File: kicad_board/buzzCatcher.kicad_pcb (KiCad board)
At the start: 2 copper layers, 63 x 100 mm, 31 parts, among them IC1 CD4043BE-NG, IC2 COM-16473, IC3 CD74HCT173E, IC4 CD4072BE, IC5 SN74LS04N, IC6 SN74LS21NE4, IC7 TS02-66-60-BK-100-SCR-D, J1 154-UL6661, J2 154-UL6661, J3 154-UL6661, J4 154-UL6661, J5 USB4130-GF-C, Q1 BS170

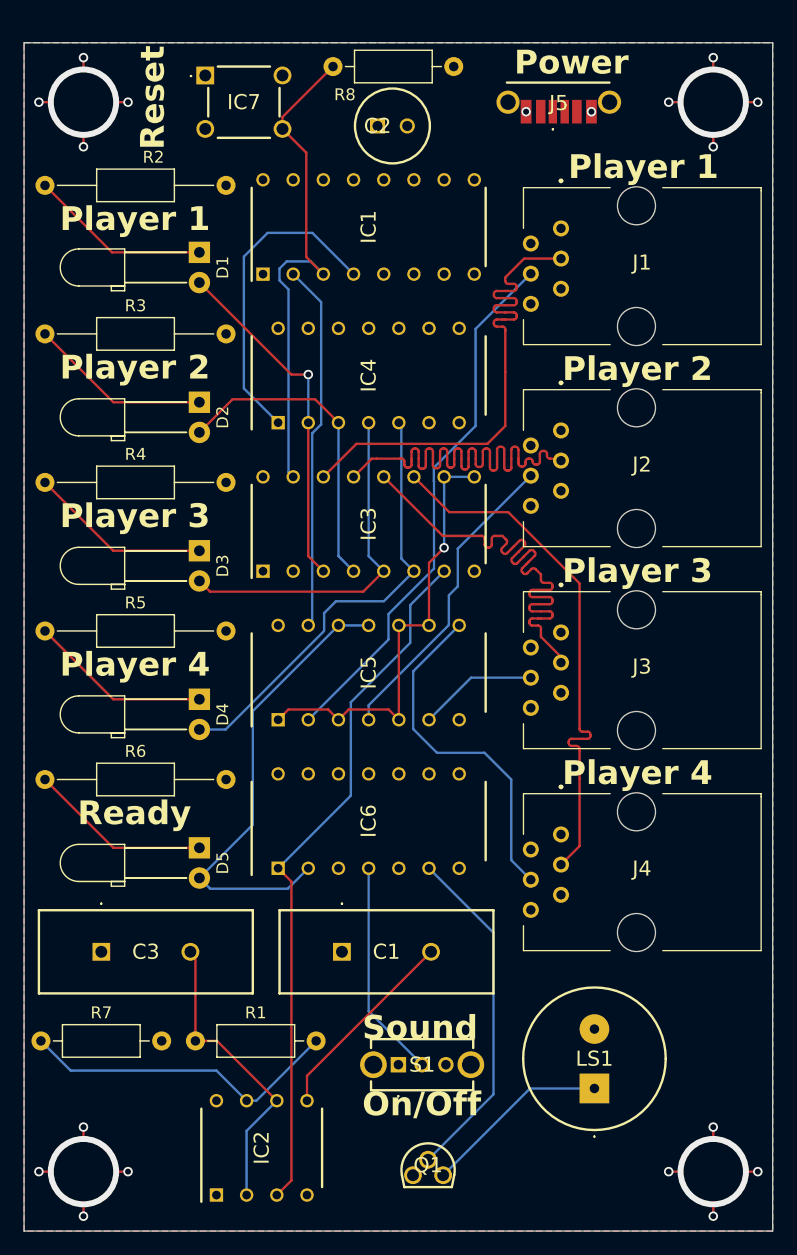
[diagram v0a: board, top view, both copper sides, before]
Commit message: Arduino version
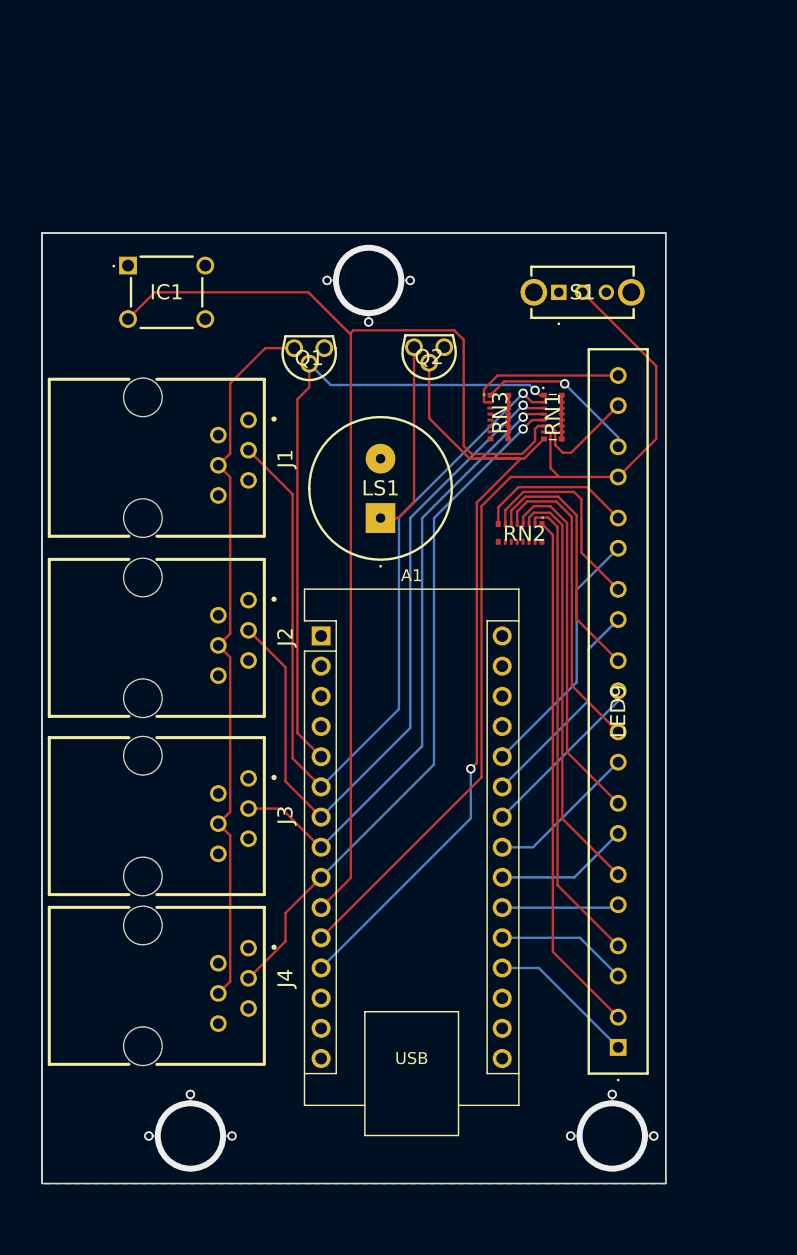
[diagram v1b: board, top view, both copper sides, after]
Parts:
- removed C1, C3: 3.3 nF, SamacSys_PCB_Library:ECWH16362RJV
- removed C2: 10 uF, SamacSys_PCB_Library:CAPPRD250W65D630H900
- removed D1, D2, D3, D4, D5: LED, LED_THT:LED_D3.0mm_Horizontal_O6.35mm_Z2.0mm
- removed IC2: COM-16473, SamacSys_PCB_Library:DIP794W53P254L959H508Q8N
- removed IC3: CD74HCT173E, SamacSys_PCB_Library:DIP794W53P254L1930H508Q16N
- removed IC4: CD4072BE, SamacSys_PCB_Library:DIP794W53P254L1930H508Q14N
- removed IC5: SN74LS04N, SamacSys_PCB_Library:DIP794W53P254L1930H508Q14N
- removed IC6: SN74LS21NE4, SamacSys_PCB_Library:DIP794W53P254L1930H508Q14N
- removed IC7: TS02-66-60-BK-100-SCR-D, SamacSys_PCB_Library:TS026660BK100SCRD
- removed J5: USB4130-GF-C, SamacSys_PCB_Library:USB4130GFC
- removed R1, R8: 110k, Resistor_THT:R_Axial_DIN0207_L6.3mm_D2.5mm_P10.16mm_Horizontal
- removed R2, R3, R4, R5, R6: 300, Resistor_THT:R_Axial_DIN0207_L6.3mm_D2.5mm_P15.24mm_Horizontal
- removed R7: 0, Resistor_THT:R_Axial_DIN0207_L6.3mm_D2.5mm_P10.16mm_Horizontal
- added A1: Arduino_Nano_v3.x, Module:Arduino_Nano, F.Cu at (75.0, 99.9)
- added LED9: SSA-LXH1025GD, SamacSys_PCB_Library:SSALXH1025GD, F.Cu at (100.0, 134.5)
- added Q2: BS170, SamacSys_PCB_Library:LM431ACZ, F.Cu at (85.4, 75.6)
- added RN1: EXB2HV103JV, SamacSys_PCB_Library:EXB2HV104JV, F.Cu at (94.5, 81.5)
- added RN2: EXB2HV121JV, SamacSys_PCB_Library:EXB2HV_1, F.Cu at (91.7, 91.3)
- added RN3: EXB2HV121JV, SamacSys_PCB_Library:EXB2HV_1, F.Cu at (90.0, 81.5)
- IC1: value CD4043BE-NG -> TS02-66-60-BK-100-SCR-D; footprint SamacSys_PCB_Library:DIP794W53P254L1930H508Q16N -> SamacSys_PCB_Library:TS026660BK100SCRD
- J1, J2, J3, J4: value 154-UL6661 -> 95501-2661; footprint SamacSys_PCB_Library:154UL6661 -> SamacSys_PCB_Library:95501-2661
- moved Q1 70.0 mm to (75.3, 75.7), turned to 180 degrees
- moved S1 66.4 mm to (95.0, 71.0)
- moved LS1 51.3 mm to (80.0, 90.0)
- moved J1 42.8 mm to (60.0, 90.0), turned to -90 degrees
- moved J2 41.8 mm to (60.0, 105.2), turned to -90 degrees
- moved J3 40.7 mm to (60.0, 120.2), turned to -90 degrees
- moved J4 39.4 mm to (60.0, 134.4), turned to -90 degrees
- moved IC1 20.5 mm to (58.8, 68.8), turned to 0 degrees
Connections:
- IC1 pad 2: /listening_state* -> unconnected-(IC1-NO_2-Pad2)
- IC1 pad 3: /reset_button -> /Button 1
- IC1 pad 4: Net-(IC1-S1) -> /Vbus_5V
- J1 pad 3: /trigger_1 -> /Trigger 1
- J1 pad 4: Net-(IC5-1Y) -> Net-(Q1-SOURCE)
- J2 pad 3: /trigger_2 -> /Trigger 2
- J2 pad 4: Net-(IC5-2Y) -> Net-(Q1-SOURCE)
- J3 pad 3: /trigger_3 -> /Trigger 3
- J3 pad 4: Net-(IC5-3Y) -> Net-(Q1-SOURCE)
- J4 pad 3: /trigger_4 -> /Trigger 4
- J4 pad 4: Net-(IC5-4Y) -> Net-(Q1-SOURCE)
- Q1 pad 2: Net-(IC6-1Y) -> /Ready
- Q1 pad 3: Net-(LS1-+) -> Net-(Q1-SOURCE)
- S1 pad 2: Net-(IC6-1C) -> /Switch 1
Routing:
- net /Button 1: track 0.00 -> 107.4 mm
- net /Switch 1: track 0.00 -> 78.5 mm
- net /Trigger 1: track 0.00 -> 73.1 mm, vias 0 -> 1
- net /Buzzer: track 0.00 -> 70.1 mm, vias 0 -> 1
- net /Trigger 2: track 0.00 -> 61.8 mm, vias 0 -> 1
- net Net-(Q1-SOURCE): track 0.00 -> 60.9 mm
- net Net-(IC2-OUT): track 59.3 -> 0.00 mm
- net /Trigger 4: track 0.00 -> 58.1 mm, vias 0 -> 1
- net /Ready: track 0.00 -> 55.2 mm, vias 0 -> 1
- net /Trigger 3: track 0.00 -> 52.6 mm, vias 0 -> 1
- net Net-(IC5-1Y): track 45.3 -> 0.00 mm
- net /trigger_4: track 44.9 -> 0.00 mm
- net /trigger_1: track 44.9 -> 0.00 mm
- net /trigger_3: track 44.8 -> 0.00 mm
- net /trigger_2: track 44.6 -> 0.00 mm
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- added copper zone on B.Cu, net /Vbus_5V
- added copper zone on F.Cu, net GND
- removed copper zone on F.Cu, net /Vbus_5V
- removed copper zone on B.Cu, net GND
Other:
- board size 63 x 100 mm -> 52.5 x 80 mm
- board text removed: "Player 1"
- board text removed: "Player 2"
- board text removed: "Player 3"
- board text removed: "Player 4"
- board text removed: "Power"
- board text removed: "Ready"
- board text removed: "Reset"
- board text removed: "Sound On/Off"
